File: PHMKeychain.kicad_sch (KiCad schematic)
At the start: 12 parts, among them J1 Conn_02x03_Odd_Even, Q1 HL2301A, U1 ATTINY85-20SU_C31540447

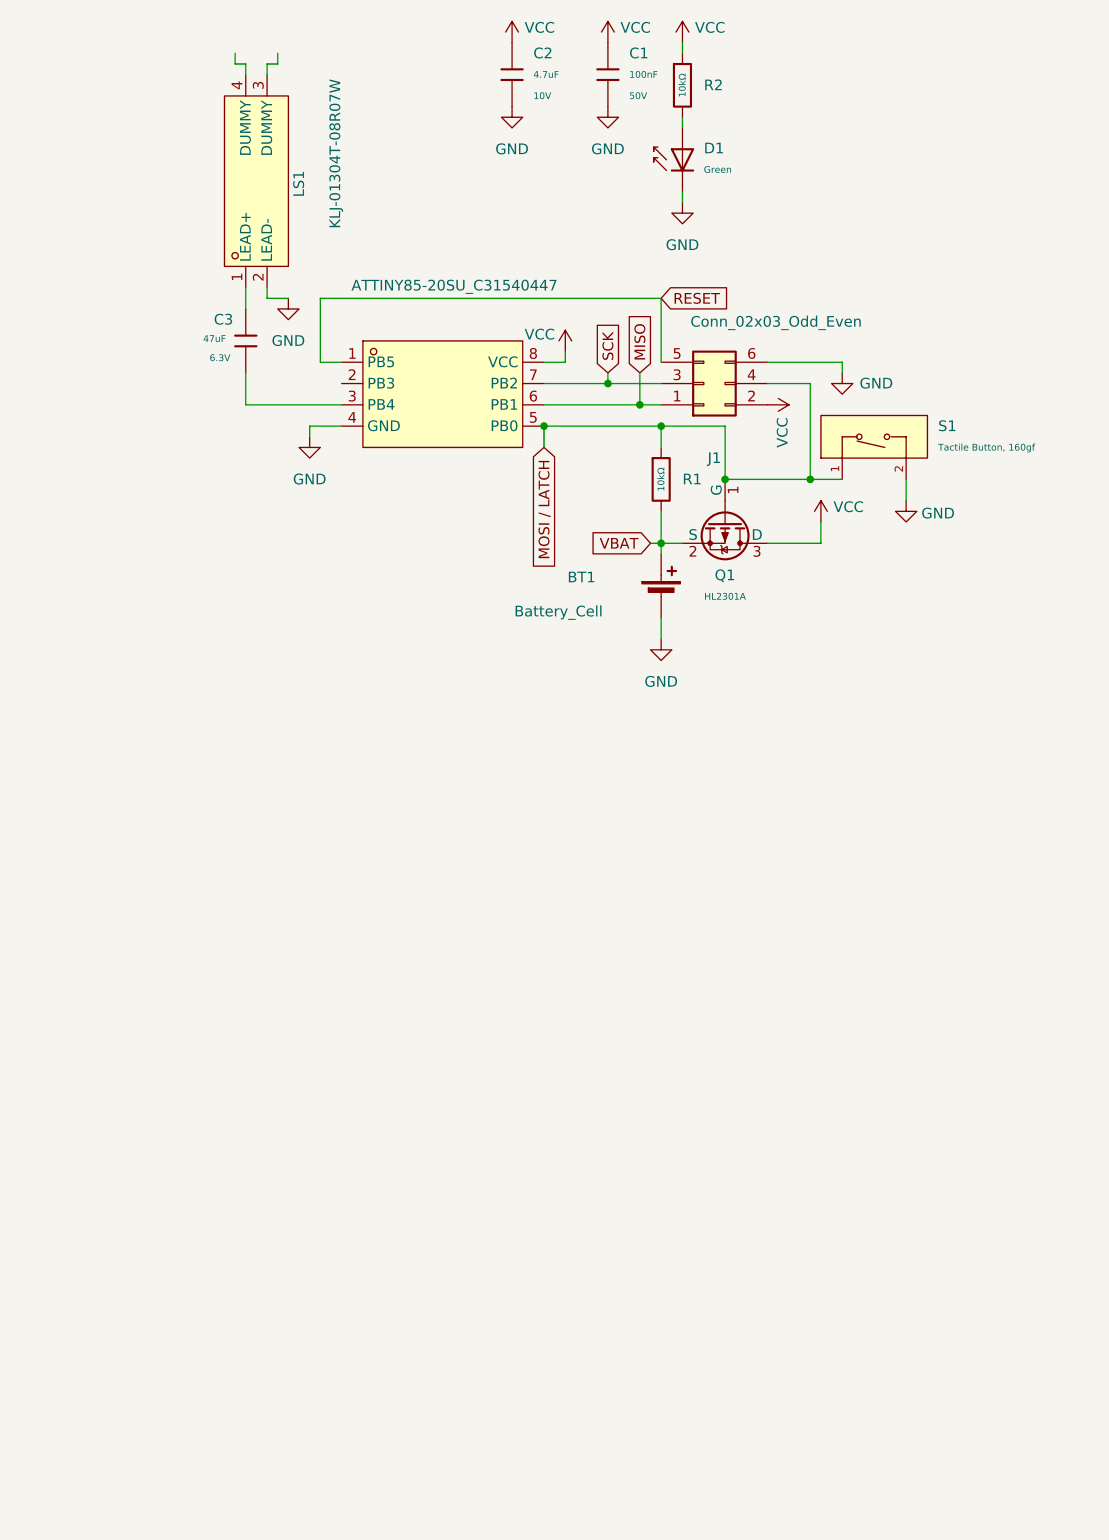
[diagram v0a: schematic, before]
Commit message: Organized
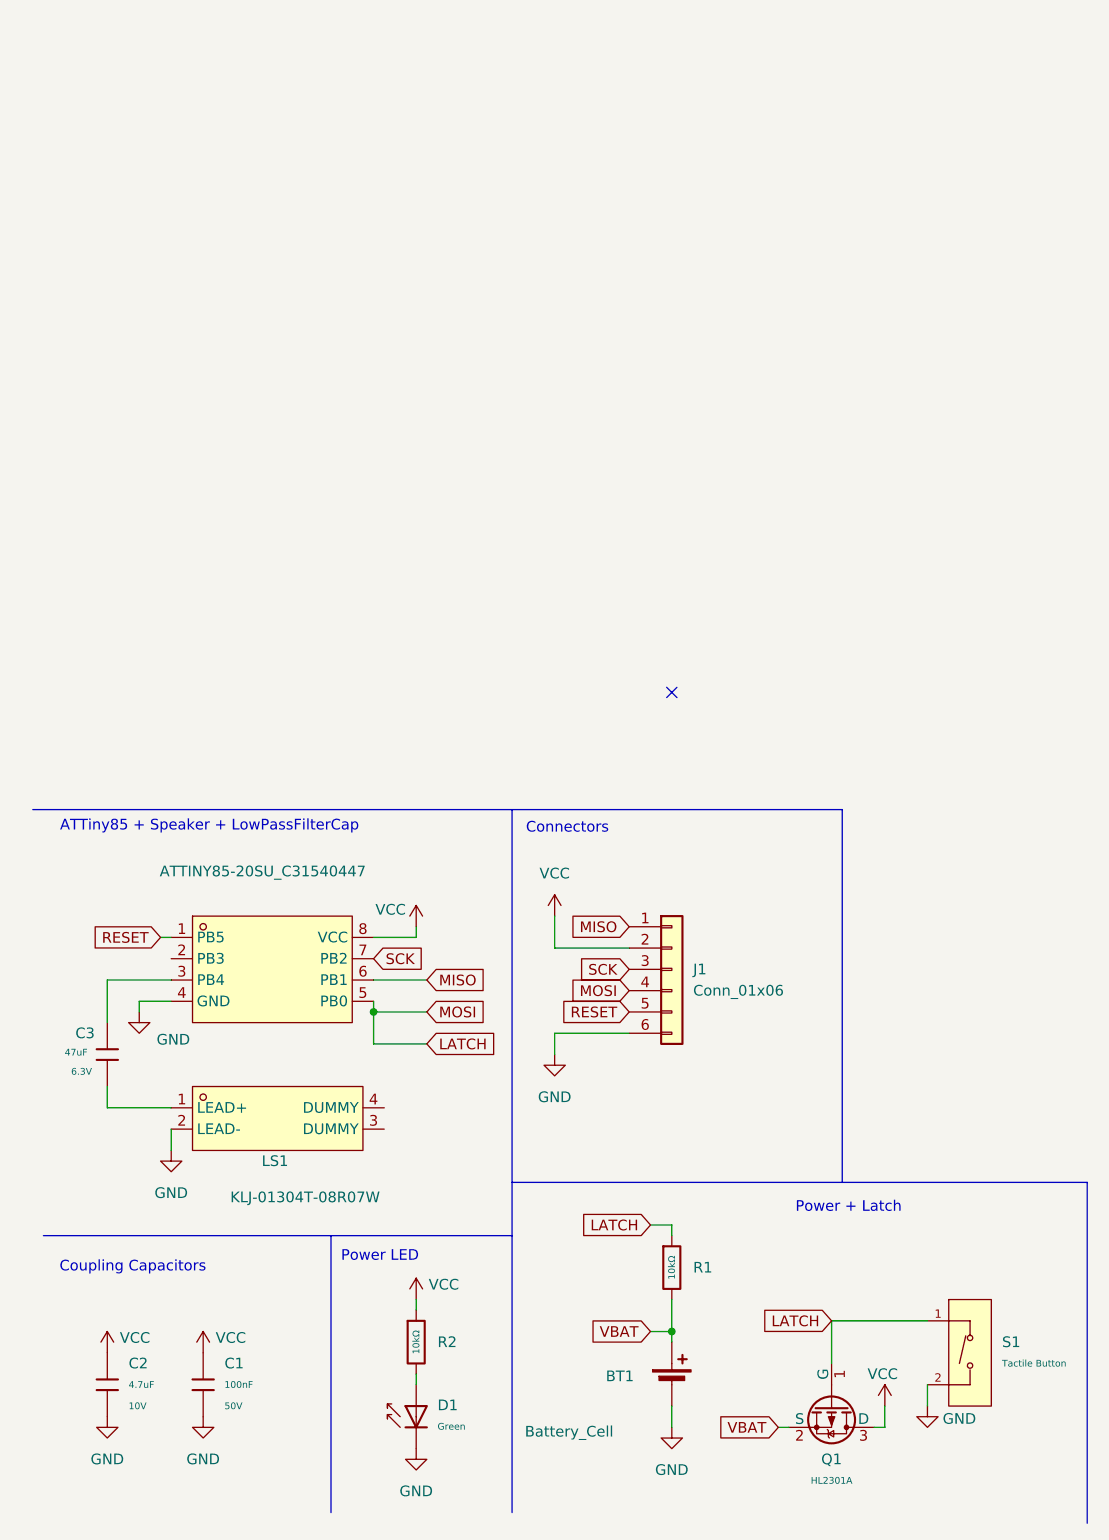
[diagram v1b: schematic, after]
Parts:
- removed J1: Conn_02x03_Odd_Even, Connector_PinHeader_1.00mm:PinHeader_1x06_P1.00mm_Vertical, symbol Connector_Generic:Conn_02x03_Odd_Even
- added J1: Conn_01x06, Connector_PinHeader_2.54mm:PinHeader_1x06_P2.54mm_Vertical, symbol Connector_Generic:Conn_01x06
- S1: value Tactile Button, 160gf -> Tactile Button
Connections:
- net GND: now also J1.6 (Pin_6)
- net MISO: now also J1.1 (Pin_1)
- net RESET: now also J1.5 (Pin_5)
- net SCK: now also J1.3 (Pin_3)
- net VCC: now also J1.2 (Pin_2)
- net at C3.1: now also U1.3 (PB4); no longer LS1.1 (LEAD+)
- net at C3.2: now also LS1.1 (LEAD+); no longer U1.3 (PB4)
- net MOSI / LATCH renamed LATCH
- net LATCH: now also J1.4 (Pin_4)
- no-connect marks 0 -> 1
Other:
- note added: "ATTiny85 + Speaker + LowPassFilterCap"
- note added: "Connectors"
- note added: "Coupling Capacitors"
- note added: "Power + Latch"
- note added: "Power LED"
- moved on the sheet: BT1, C1, C2, C3, D1, LS1, Q1, R1, R2, S1
